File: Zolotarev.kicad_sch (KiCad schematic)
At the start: 176 parts, among them J1 RF_IN, J2 RF_OUT, J3 Conn_02x05_Odd_Even, K1 G5LE-1, K10 G5LE-1, K11 G5LE-1, K12 G5LE-1, K13 G5LE-1, K14 G5LE-1, K2 G5LE-1, K3 G5LE-1, K4 G5LE-1, K5 G5LE-1, K6 G5LE-1, K7 G5LE-1, K8 G5LE-1, K9 G5LE-1

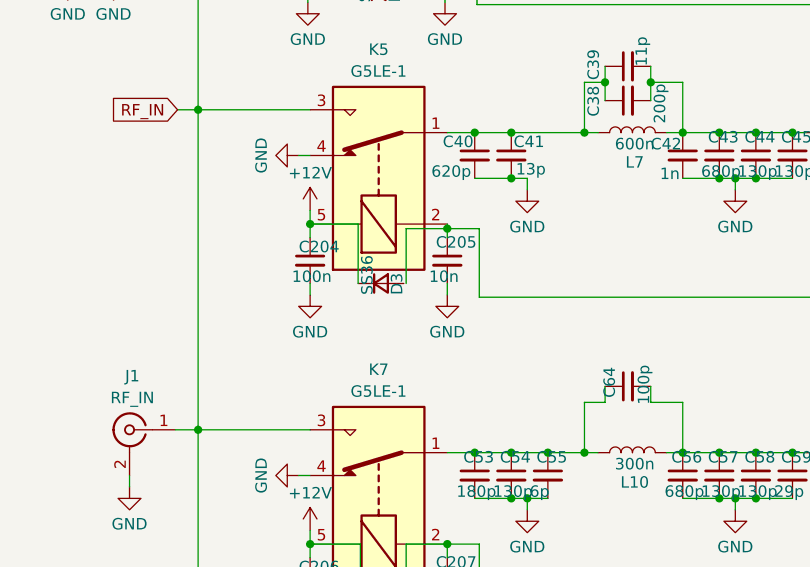
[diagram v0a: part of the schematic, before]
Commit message: 3 bands over 7
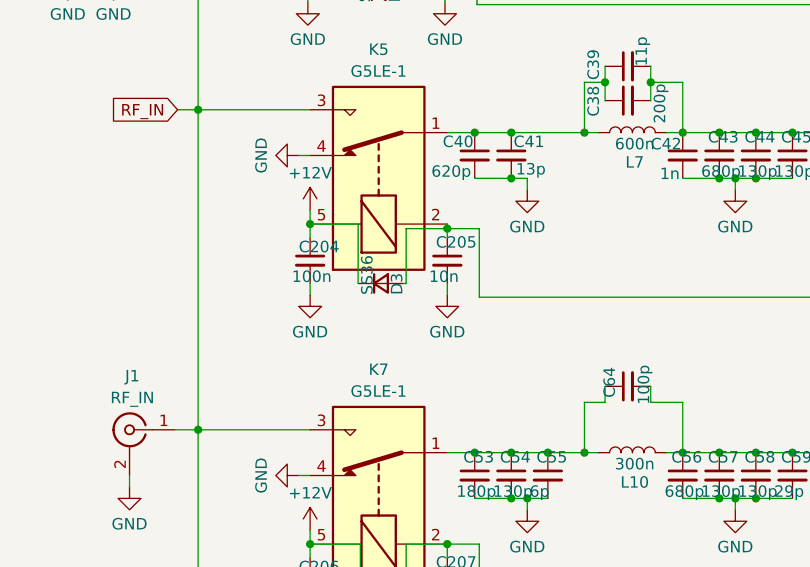
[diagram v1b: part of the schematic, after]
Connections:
- net 60+40m: now also D3.2 (A)
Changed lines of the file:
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@@
+	(wire
+		(pts
+			(xy 51.816 107.188) (xy 52.07 107.188)
+		)
+		(stroke
+			(width 0)
+			(type default)
+		)
+	)
 	(wire
 		(pts
